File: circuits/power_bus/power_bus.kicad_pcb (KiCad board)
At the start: 2 copper layers, 105.4 x 57.2 mm, 25 parts, among them P1 CONN_02X03, P10 CONN_01X03, P11 CONN_01X03, P12 CONN_01X03, P13 CONN_01X03, P14 CONN_01X03, P15 CONN_01X03, P16 CONN_01X03, P17 CONN_01X03, P18 CONN_01X02, P19 CONN_01X03, P2 CONN_01X03, P20 CONN_01X03, P21 CONN_01X03, P22 CONN_01X03, P3 CONN_01X03, P4 CONN_01X03, P5 CONN_01X03, P6 CONN_01X01, P7 CONN_01X01, P8 CONN_01X01, P9 CONN_01X01, U1 CD4067

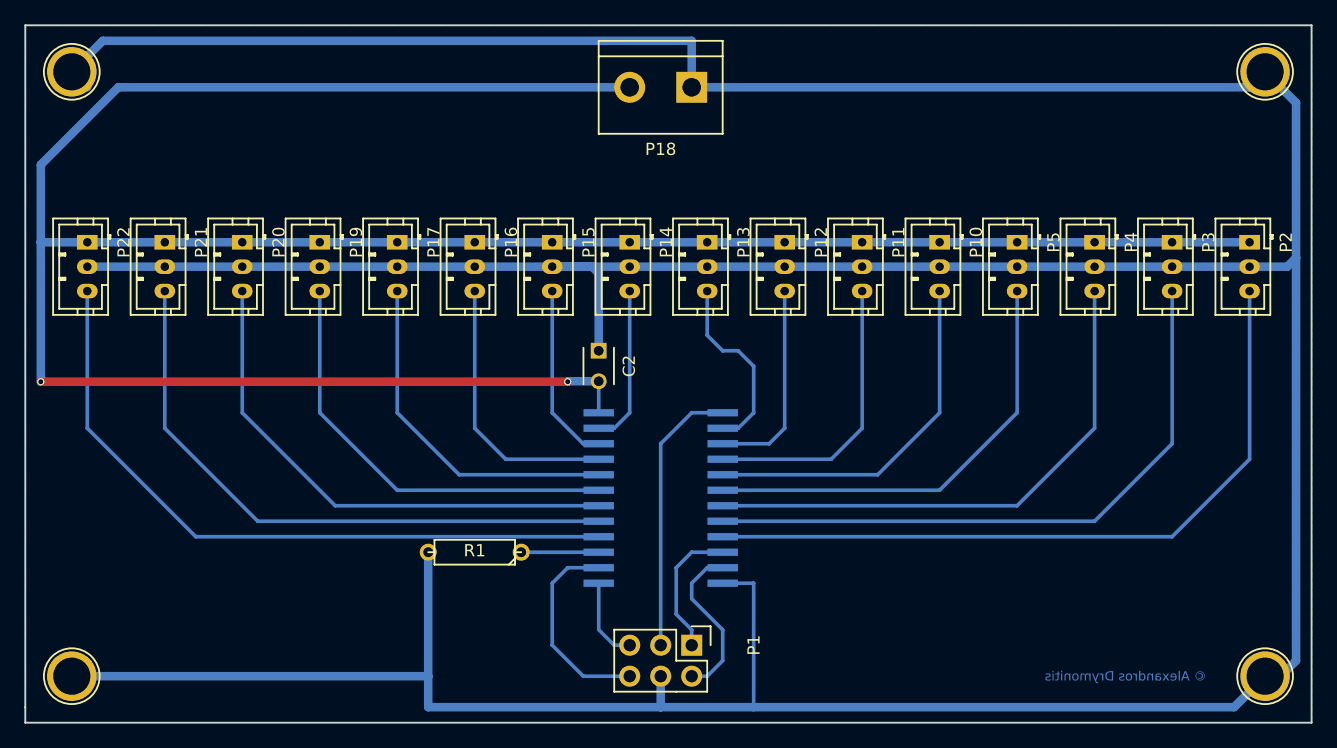
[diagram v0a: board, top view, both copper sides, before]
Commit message: Update circuits
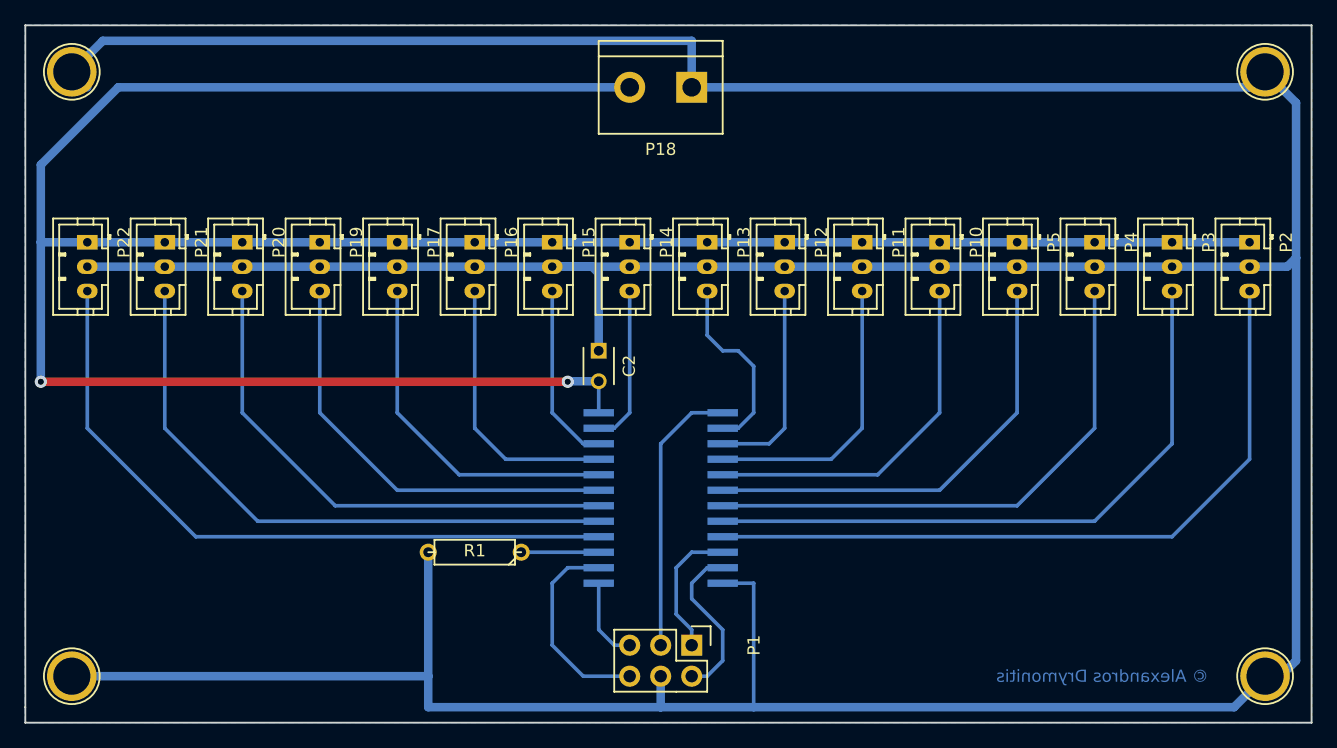
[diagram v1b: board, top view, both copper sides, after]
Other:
- net class Default: via_dia 0.6 -> 1; via_drill 0.4 -> 0.5
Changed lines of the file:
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@@
-(kicad_pcb (version 4) (host pcbnew 4.0.2+dfsg1-2~bpo8+1-stable)
+(kicad_pcb (version 4) (host pcbnew 4.0.6+dfsg1-1)
   (general
     (links 64)
     (no_connects 0)
-    (area 91.364999 71.044999 196.925001 128.345001)
+    (area 90.216667 70.145 198.073334 128.345001)
     (thickness 1.6)
     (drawings 6)
@@
   (title_block
     (title "Modular Synthesizer Power Bus")
-    (date 2017-07-12)
+    (date 2017-11-01)
+    (rev 1)
     (company "Alexandros Drymonitis")
   )
@@
     (segment_width 0.2)
     (edge_width 0.15)
-    (via_size 0.6)
-    (via_drill 0.4)
+    (via_size 1)
+    (via_drill 0.5)
     (via_min_size 0.5)
     (via_min_drill 0.3)
@@
     (visible_elements FFFFFF7F)
     (pcbplotparams
-      (layerselection 0x00030_80000001)
+      (layerselection 0x010f0_80000001)
       (usegerberextensions false)
       (excludeedgelayer true)
@@
       (outputformat 1)
       (mirror false)
-      (drillshape 1)
+      (drillshape 0)
       (scaleselection 1)
-      (outputdirectory ""))
+      (outputdirectory ../../../../Documents/kicad/3dPd/power_bus/svg_files/))
   )
   (net 0 "")
@@
     (clearance 0.2)
     (trace_width 0.3)
-    (via_dia 0.6)
-    (via_drill 0.4)
+    (via_dia 1)
+    (via_drill 0.5)
     (uvia_dia 0.3)
     (uvia_drill 0.1)
@@
       (net 1 GND))
   )
-  (gr_text "© Alexandros Drymonitis" (at 181.61 124.46) (layer B.Cu)
-    (effects (font (size 0.762 0.762) (thickness 0.1905)) (justify mirror))
+  (gr_text "© Alexandros Drymonitis" (at 179.705 124.46) (layer B.Cu)
+    (effects (font (size 1 1) (thickness 0.1905)) (justify mirror))
   )
   (gr_line (start 196.85 128.27) (end 196.85 71.12) (angle 90) (layer Edge.Cuts) (width 0.15))
@@
   (segment (start 138.43 100.29) (end 135.93 100.29) (width 0.7) (layer B.Cu) (net 2))
   (segment (start 92.71 100.33) (end 92.71 88.9) (width 0.7) (layer B.Cu) (net 2))
-  (via (at 92.71 100.33) (size 0.6) (drill 0.4) (layers F.Cu B.Cu) (net 2))
+  (via (at 92.71 100.33) (size 1) (drill 0.5) (layers F.Cu B.Cu) (net 2))
   (segment (start 135.89 100.33) (end 92.71 100.33) (width 0.7) (layer F.Cu) (net 2))
-  (via (at 135.89 100.33) (size 0.6) (drill 0.4) (layers F.Cu B.Cu) (net 2))
+  (via (at 135.89 100.33) (size 1) (drill 0.5) (layers F.Cu B.Cu) (net 2))
   (segment (start 135.93 100.29) (end 135.89 100.33) (width 0.7) (layer B.Cu) (net 2))
   (segment (start 140.97 76.2) (end 99.06 76.2) (width 0.7) (layer B.Cu) (net 2))
+  (segment (start 92.71 82.55) (end 92.71 88.9) (width 0.7) (layer B.Cu) (net 2))
   (segment (start 99.06 76.2) (end 92.71 82.55) (width 0.7) (layer B.Cu) (net 2))
-  (segment (start 92.71 82.55) (end 92.71 88.9) (width 0.7) (layer B.Cu) (net 2))
   (segment (start 92.71 88.9) (end 96.52 88.9) (width 0.7) (layer B.Cu) (net 2))
   (segment (start 138.43 100.29) (end 138.43 102.87) (width 0.3) (layer B.Cu) (net 2))
@@
     (polygon
       (pts
-        (xy 196.85 128.27) (xy 91.44 128.27) (xy 91.44 71.12) (xy 196.85 71.12) (xy 196.85 128.27)
+        (xy 196.85 128.27) (xy 91.44 128.27) (xy 91.44 71.12) (xy 196.85 71.12)
       )
     )
